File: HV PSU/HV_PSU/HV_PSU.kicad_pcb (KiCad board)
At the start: 2 copper layers, 200 x 80 mm, 105 parts, among them J1 Screw_Terminal_01x07, J13 MountingHole_Pad, J2 AC_HV_1, J3 AC_HV_2, J4 MountingHole_Pad, J5 AC_HV_2, Q1 2N7002, Q2 IRFS4227, Q3 IRFS4227, T1 UY12, U1 L7812, U2 TPS2814D

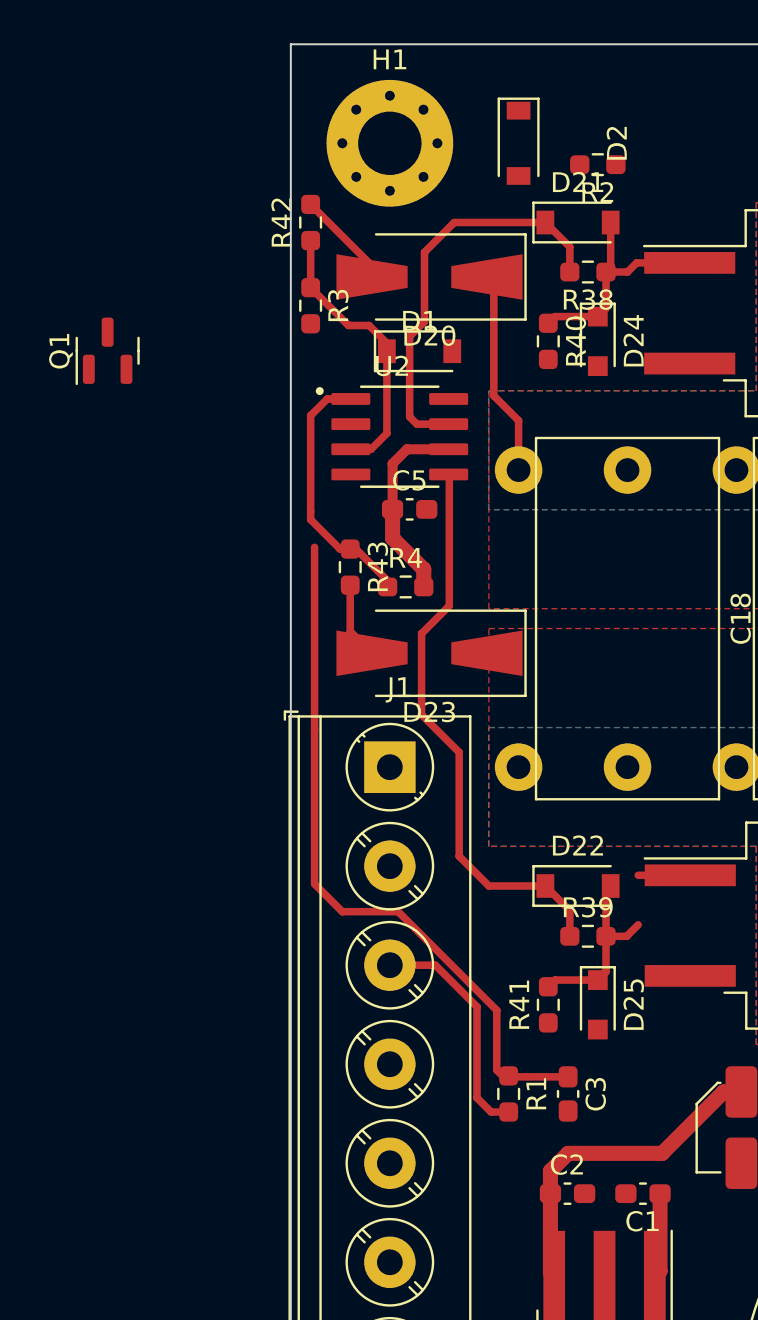
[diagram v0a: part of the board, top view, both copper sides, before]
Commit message: Some routing done
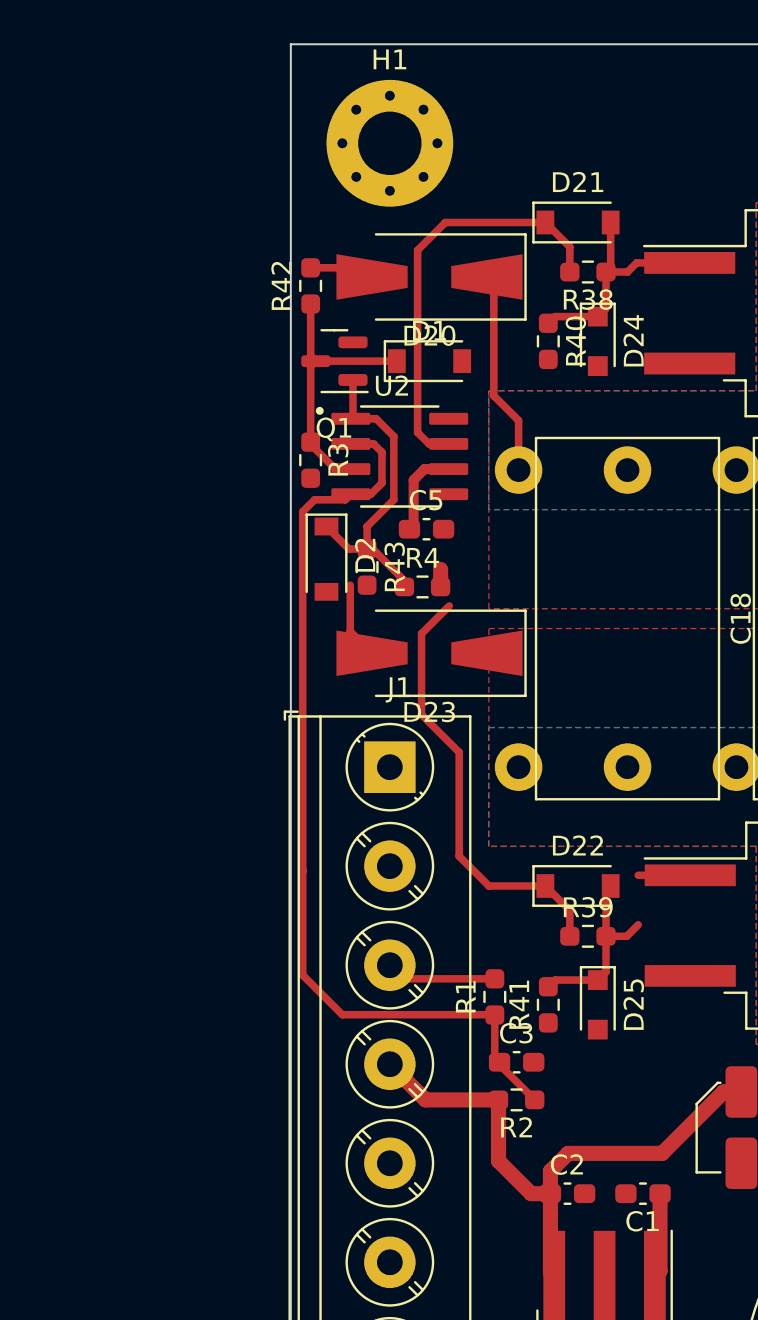
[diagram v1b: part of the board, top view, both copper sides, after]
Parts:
- moved R2 47.4 mm to (11.4, 73.3)
- moved D2 23.1 mm to (1.80, 46.0)
- moved Q1 11.5 mm to (2.20, 36.0), turned to 180 degrees
- moved R3 7.80 mm to (1.00, 41.0)
- moved R1 4.95 mm to (10.3, 68.1), turned to 90 degrees
- moved R42 3.20 mm to (1.00, 32.2)
- moved C3 3.05 mm to (11.4, 71.4), turned to 0 degrees
- moved C5 1.31 mm to (6.85, 44.5)
- moved U2 1.00 mm to (5.50, 40.8)
- moved R4 0.85 mm to (6.65, 47.4)
- moved R43 0.85 mm to (3.85, 46.4)
- moved D1 0.71 mm to (7.00, 36.0)
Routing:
- net Net-(C3-Pad1): track 35.6 -> 47.1 mm
- net +12V: track 26.7 -> 34.8 mm
- net Net-(D22-Pad1): track 28.7 -> 22.1 mm
- net Net-(J1-Pad3): track 11.8 -> 5.71 mm
- net Net-(D2-Pad1): track 13.1 -> 16.2 mm
- net Net-(D20-Pad2): track 4.95 -> 3.29 mm
- net Net-(D21-Pad1): track 20.5 -> 21.1 mm
